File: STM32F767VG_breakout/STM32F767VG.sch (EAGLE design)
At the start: 42 parts, among them IC1 STM32F767VGT6, IC3 LD117AS33TR, X4 8MHz, X5 32.768kHz

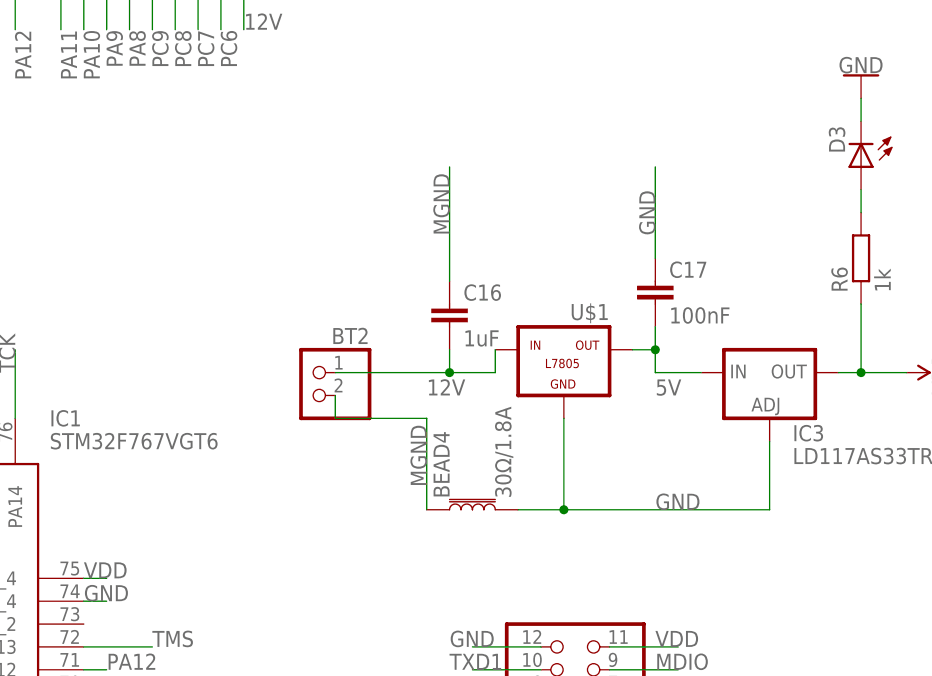
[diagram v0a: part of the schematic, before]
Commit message: Incorporated April 6 Comments
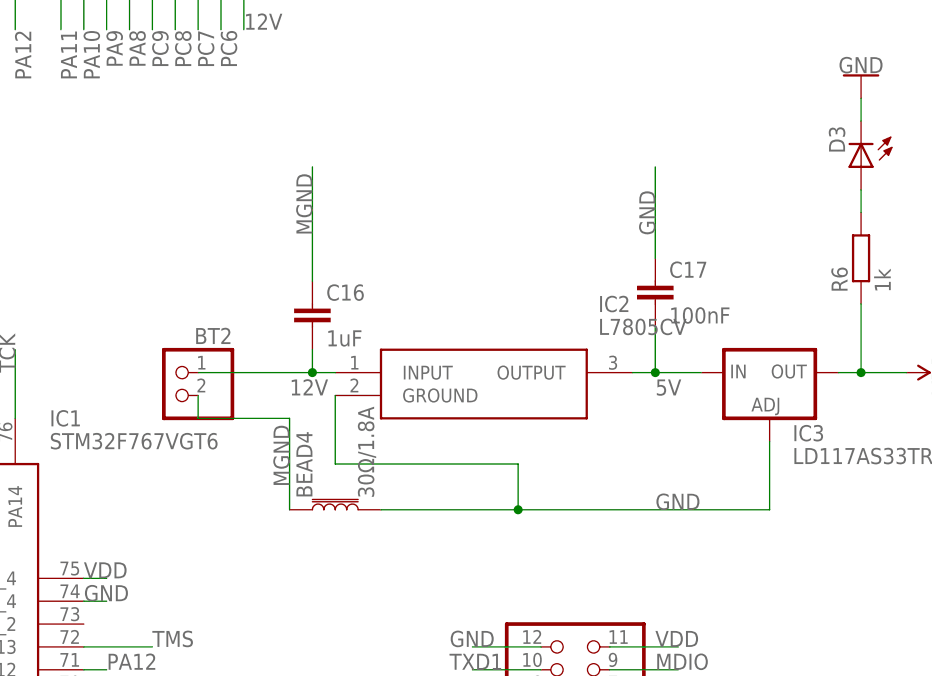
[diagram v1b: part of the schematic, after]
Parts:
- removed U$1: -L7805, tango:-L7805
- added IC2: L7805CV, L7805CV:L7805CV
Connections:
- net 12V: now also IC2.INPUT; no longer U$1.IN
- net 5V: now also IC2.OUTPUT; no longer U$1.OUT
- net GND: now also IC2.GROUND; no longer U$1.GND
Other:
- moved on the sheet: BEAD4, BT2, C16
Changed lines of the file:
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@@
 <part name="C1" library="eagle-ltspice" library_urn="urn:adsk.eagle:library:217" deviceset="C" device="" package3d_urn="urn:adsk.eagle:package:13265/1" value="100nF"/>
 <part name="BT2" library="pinhead" library_urn="urn:adsk.eagle:library:325" deviceset="PINHD-1X2" device="" package3d_urn="urn:adsk.eagle:package:22435/2"/>
-<part name="U$1" library="tango" deviceset="-L7805" device=""/>
+<part name="IC2" library="L7805CV" deviceset="L7805CV" device=""/>
 </parts>
 <sheets>
@@
 <instance part="IC3" gate="G$1" x="152.4" y="22.86"/>
 <instance part="SUPPLY15" gate="VDD" x="167.64" y="22.86" rot="R270"/>
-<instance part="BEAD4" gate="G$1" x="119.38" y="7.62" rot="R90"/>
-<instance part="C16" gate="G$1" x="116.84" y="30.48"/>
+<instance part="BEAD4" gate="G$1" x="104.14" y="7.62" rot="R90"/>
+<instance part="C16" gate="G$1" x="101.6" y="30.48"/>
 <instance part="C17" gate="G$1" x="139.7" y="33.02"/>
 <instance part="R6" gate="G$1" x="162.56" y="35.56" rot="R90"/>
@@
 <instance part="GND4" gate="1" x="-12.7" y="40.64" rot="R90"/>
 <instance part="C1" gate="G$1" x="-20.32" y="-78.74"/>
-<instance part="BT2" gate="G$1" x="101.6" y="20.32" rot="MR0"/>
-<instance part="U$1" gate="G$1" x="129.54" y="22.86"/>
+<instance part="BT2" gate="G$1" x="86.36" y="20.32" rot="MR0"/>
+<instance part="IC2" gate="G$1" x="104.14" y="22.86"/>
 </instances>
 <busses>
@@
 <pinref part="BEAD4" gate="G$1" pin="2"/>
 <pinref part="IC3" gate="G$1" pin="ADJ"/>
-<wire x1="124.46" y1="7.62" x2="129.54" y2="7.62" width="0.1524" layer="91"/>
-<wire x1="129.54" y1="7.62" x2="152.4" y2="7.62" width="0.1524" layer="91"/>
+<wire x1="109.22" y1="7.62" x2="124.46" y2="7.62" width="0.1524" layer="91"/>
+<wire x1="124.46" y1="7.62" x2="152.4" y2="7.62" width="0.1524" layer="91"/>
 <wire x1="152.4" y1="7.62" x2="152.4" y2="15.24" width="0.1524" layer="91"/>
-<wire x1="129.54" y1="17.78" x2="129.54" y2="7.62" width="0.1524" layer="91"/>
-<junction x="129.54" y="7.62"/>
 <label x="139.7" y="7.62" size="1.778" layer="95"/>
-<pinref part="U$1" gate="G$1" pin="GND"/>
+<pinref part="IC2" gate="G$1" pin="GROUND"/>
+<wire x1="104.14" y1="20.32" x2="104.14" y2="12.7" width="0.1524" layer="91"/>
+<wire x1="104.14" y1="12.7" x2="124.46" y2="12.7" width="0.1524" layer="91"/>
+<wire x1="124.46" y1="12.7" x2="124.46" y2="7.62" width="0.1524" layer="91"/>
+<junction x="124.46" y="7.62"/>
 </segment>
 <segment>
@@
 <net name="12V" class="0">
 <segment>
-<label x="114.3" y="20.32" size="1.778" layer="95"/>
+<label x="99.06" y="20.32" size="1.778" layer="95"/>
 <pinref part="C16" gate="G$1" pin="2"/>
-<wire x1="116.84" y1="25.4" x2="116.84" y2="22.86" width="0.1524" layer="91"/>
+<wire x1="101.6" y1="25.4" x2="101.6" y2="22.86" width="0.1524" layer="91"/>
 <pinref part="BT2" gate="G$1" pin="1"/>
-<wire x1="104.14" y1="22.86" x2="116.84" y2="22.86" width="0.1524" layer="91"/>
-<pinref part="U$1" gate="G$1" pin="IN"/>
-<wire x1="121.92" y1="25.4" x2="121.92" y2="22.86" width="0.1524" layer="91"/>
-<wire x1="121.92" y1="22.86" x2="116.84" y2="22.86" width="0.1524" layer="91"/>
-<junction x="116.84" y="22.86"/>
+<wire x1="88.9" y1="22.86" x2="101.6" y2="22.86" width="0.1524" layer="91"/>
+<pinref part="IC2" gate="G$1" pin="INPUT"/>
+<wire x1="104.14" y1="22.86" x2="101.6" y2="22.86" width="0.1524" layer="91"/>
+<junction x="101.6" y="22.86"/>
 </segment>
 <segment>
@@
 <label x="139.7" y="20.32" size="1.778" layer="95"/>
 <wire x1="139.7" y1="22.86" x2="144.78" y2="22.86" width="0.1524" layer="91"/>
-<wire x1="139.7" y1="27.94" x2="139.7" y2="25.4" width="0.1524" layer="91"/>
 <pinref part="C17" gate="G$1" pin="2"/>
-<pinref part="U$1" gate="G$1" pin="OUT"/>
-<wire x1="139.7" y1="25.4" x2="139.7" y2="22.86" width="0.1524" layer="91"/>
-<wire x1="137.16" y1="25.4" x2="139.7" y2="25.4" width="0.1524" layer="91"/>
-<junction x="139.7" y="25.4"/>
+<wire x1="139.7" y1="27.94" x2="139.7" y2="22.86" width="0.1524" layer="91"/>
+<pinref part="IC2" gate="G$1" pin="OUTPUT"/>
+<wire x1="137.16" y1="22.86" x2="139.7" y2="22.86" width="0.1524" layer="91"/>
+<junction x="139.7" y="22.86"/>
 </segment>
 </net>
@@
 <segment>
 <pinref part="BEAD4" gate="G$1" pin="1"/>
-<wire x1="114.3" y1="17.78" x2="114.3" y2="7.62" width="0.1524" layer="91"/>
-<label x="114.3" y="10.16" size="1.778" layer="95" rot="R90"/>
+<wire x1="99.06" y1="17.78" x2="99.06" y2="7.62" width="0.1524" layer="91"/>
+<label x="99.06" y="10.16" size="1.778" layer="95" rot="R90"/>
 <pinref part="BT2" gate="G$1" pin="2"/>
-<wire x1="114.3" y1="17.78" x2="104.14" y2="17.78" width="0.1524" layer="91"/>
-<wire x1="104.14" y1="17.78" x2="104.14" y2="20.32" width="0.1524" layer="91"/>
+<wire x1="99.06" y1="17.78" x2="88.9" y2="17.78" width="0.1524" layer="91"/>
+<wire x1="88.9" y1="17.78" x2="88.9" y2="20.32" width="0.1524" layer="91"/>
 </segment>
 <segment>
 <pinref part="C16" gate="G$1" pin="1"/>
-<wire x1="116.84" y1="33.02" x2="116.84" y2="45.72" width="0.1524" layer="91"/>
-<label x="116.84" y="38.1" size="1.778" layer="95" rot="R90"/>
-</segment>
-</net>
+<wire x1="101.6" y1="33.02" x2="101.6" y2="45.72" width="0.1524" layer="91"/>
+<label x="101.6" y="38.1" size="1.778" layer="95" rot="R90"/>
+</segment>
+</net>
